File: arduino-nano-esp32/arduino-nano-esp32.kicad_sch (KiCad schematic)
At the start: 1 part

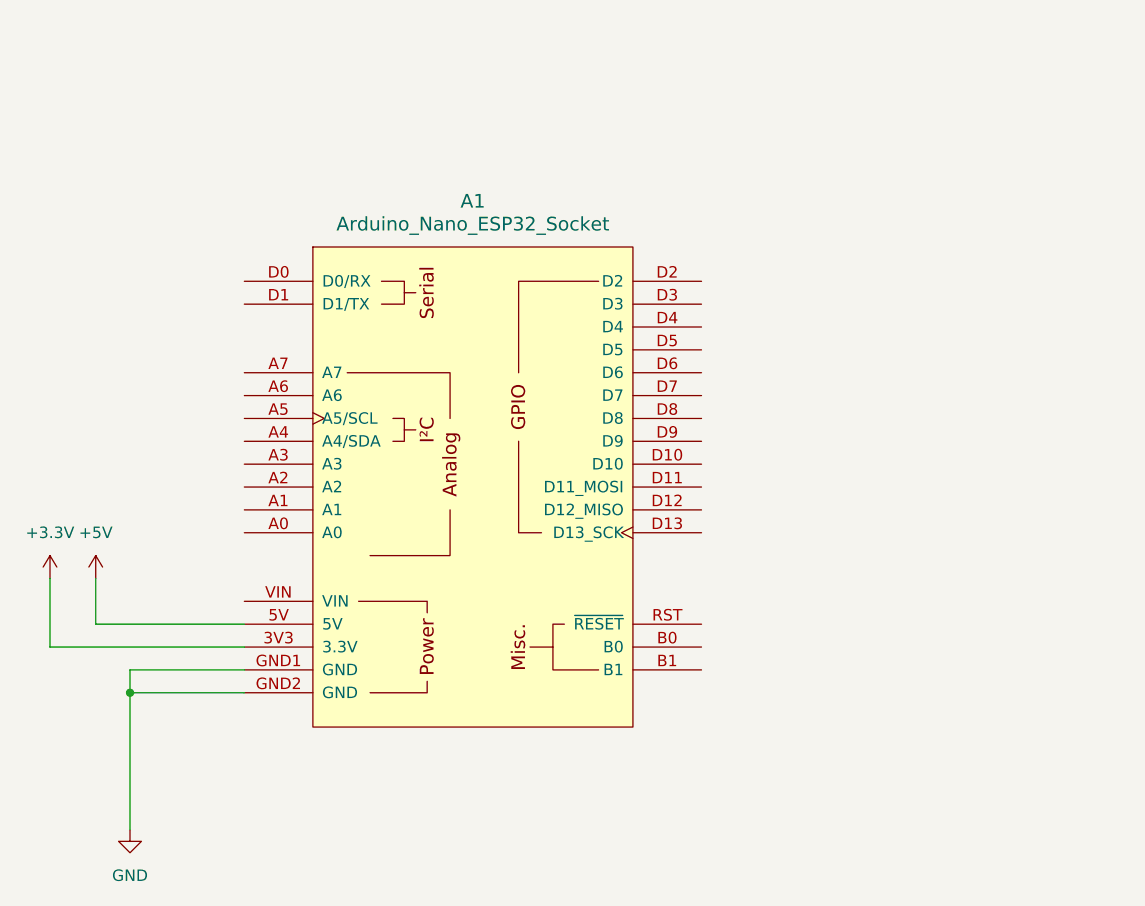
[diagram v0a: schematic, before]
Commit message: symbol lib
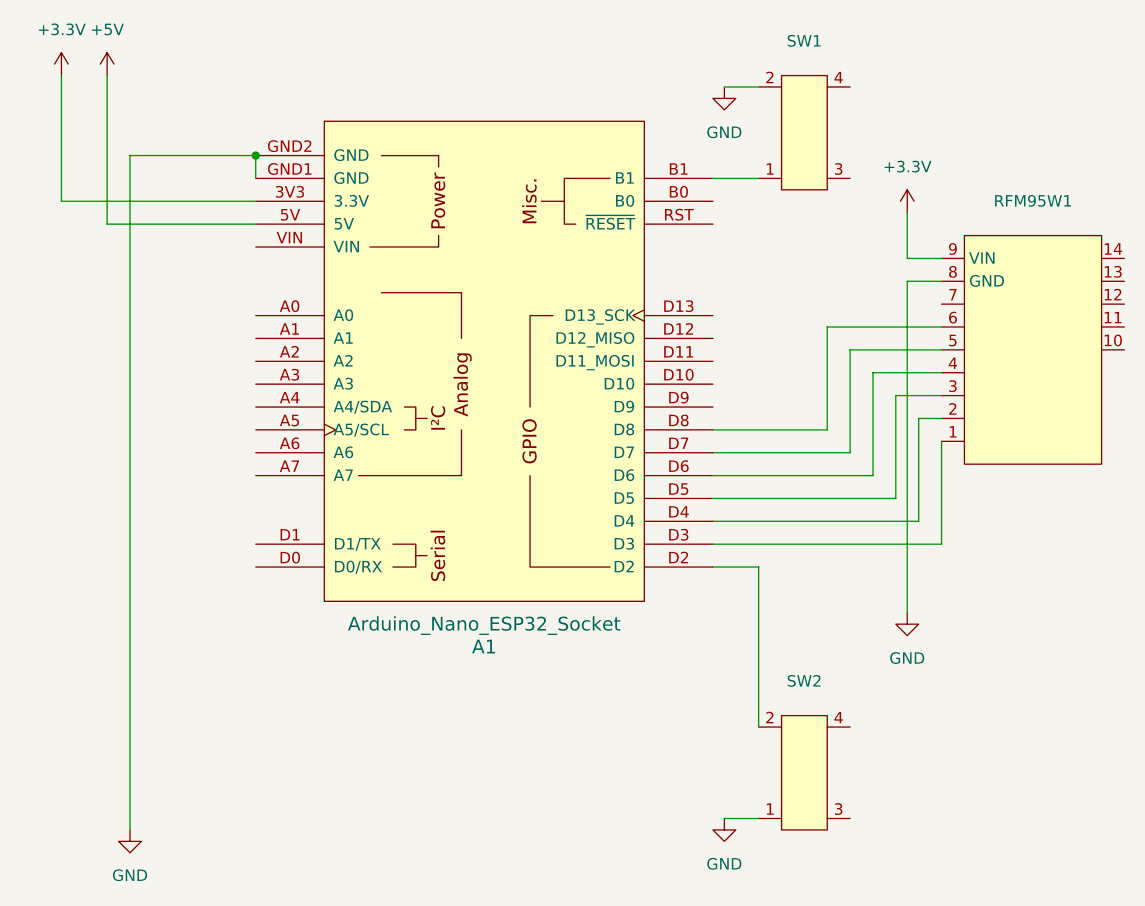
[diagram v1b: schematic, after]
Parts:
- added RFM95W1: ~, maciek-lib:lora-adafruit, symbol maciek-symbols:adafruit-rfm95w
- added SW1, SW2: ~, maciek-lib:3x4 switch, symbol maciek-symbols:3x4_switch
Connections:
- net +3.3V: now also RFM95W1.9 (VIN)
- net GND: now also RFM95W1.8 (GND), SW1.2, SW2.1
- net at A1.B1: now also SW1.1
- net at A1.D2: now also SW2.2
- net at A1.D3: now also RFM95W1.1
- net at A1.D4: now also RFM95W1.2
- net at A1.D5: now also RFM95W1.3
- net at A1.D6: now also RFM95W1.4
- net at A1.D7: now also RFM95W1.5
- net at A1.D8: now also RFM95W1.6
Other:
- moved on the sheet: A1
